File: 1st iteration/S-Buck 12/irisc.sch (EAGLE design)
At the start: 14 parts, among them U1 LM2695MH

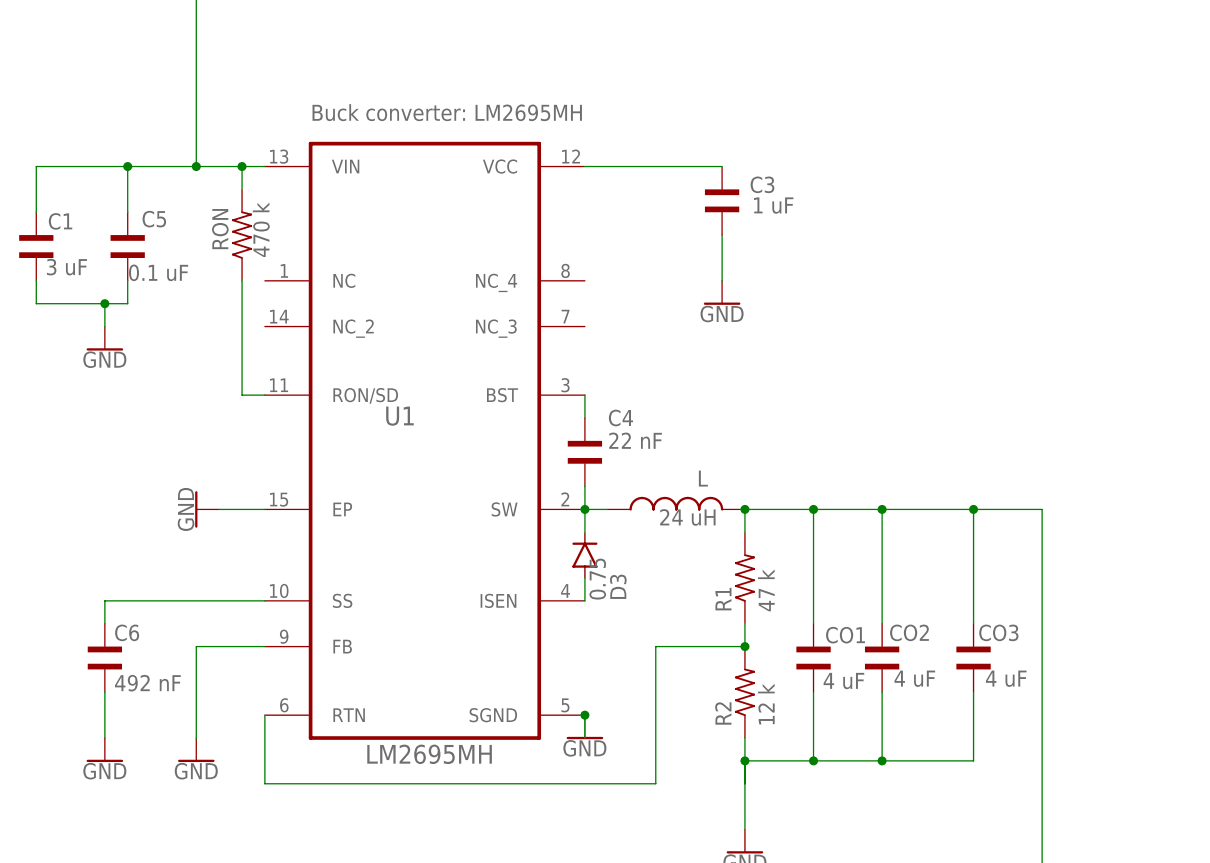
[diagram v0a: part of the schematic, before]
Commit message: Update irisc.sch
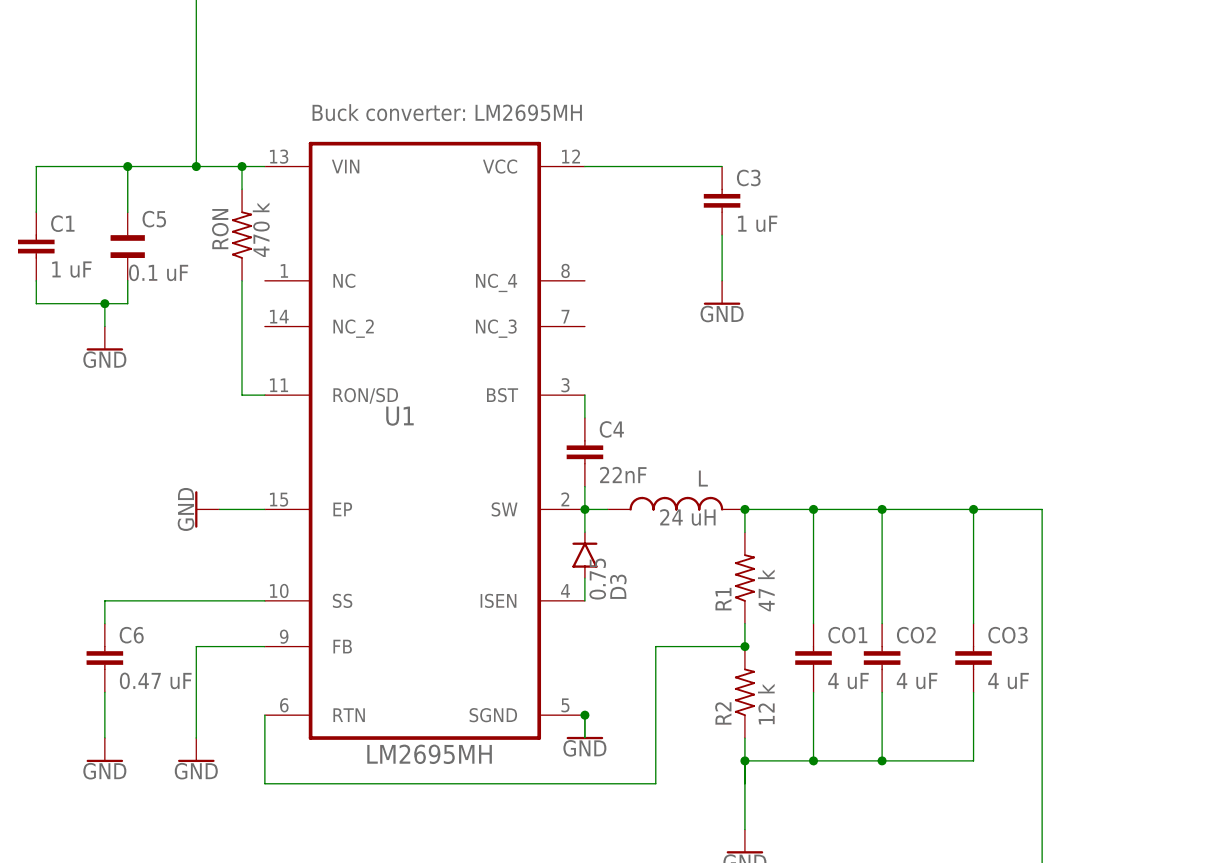
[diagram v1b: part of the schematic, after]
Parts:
- C1: value 3 uF -> 1 uF; device Wurth_Elektronik_Passive_Capacitors_rev18b:WCAP-CSGP_0805_885012006082_REFLOW -> eagle-ltspice:CC1210; SPICEPREFIX C -> (none)
- C3: device Wurth_Elektronik_Passive_Capacitors_rev18b:WCAP-CSGP_0805_885012006018_WAVE -> eagle-ltspice:CC1210; SPICEPREFIX C -> (none)
- C4: value 22 nF -> 22nF; device Wurth_Elektronik_Passive_Capacitors_rev18b:WCAP-CSGP_0805_885012006018_WAVE -> eagle-ltspice:CC1206; SPICEPREFIX C -> (none)
- C6: value 492 nF -> 0.47 uF; device Wurth_Elektronik_Passive_Capacitors_rev18b:WCAP-CSGP_0805_885012006018_WAVE -> eagle-ltspice:CC1210; SPICEPREFIX C -> (none)
- CO1, CO2, CO3: device Wurth_Elektronik_Passive_Capacitors_rev18b:WCAP-CSGP_0805_885012006018_WAVE -> eagle-ltspice:CC1812; SPICEPREFIX C -> (none)
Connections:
- net 12V: now also CO1.1, CO2.1, CO3.1; no longer CO1.2, CO2.2, CO3.2
- net GND: now also C1.2, C3.2, C6.2, CO1.2, CO2.2, CO3.2; no longer C1.1, C3.1, C6.1, CO1.1, CO2.1, CO3.1
- net N$124: now also C3.1; no longer C3.2
- net N$125: now also C4.1; no longer C4.2
- net N$126: now also C4.2; no longer C4.1
- net N$128: now also C6.1; no longer C6.2
- net VCC: now also C1.1; no longer C1.2

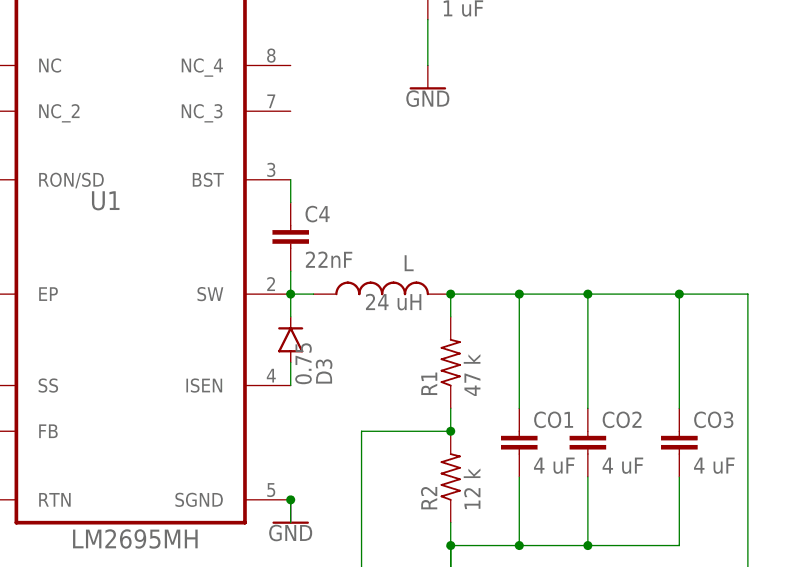
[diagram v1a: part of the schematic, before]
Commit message: Update irisc.sch
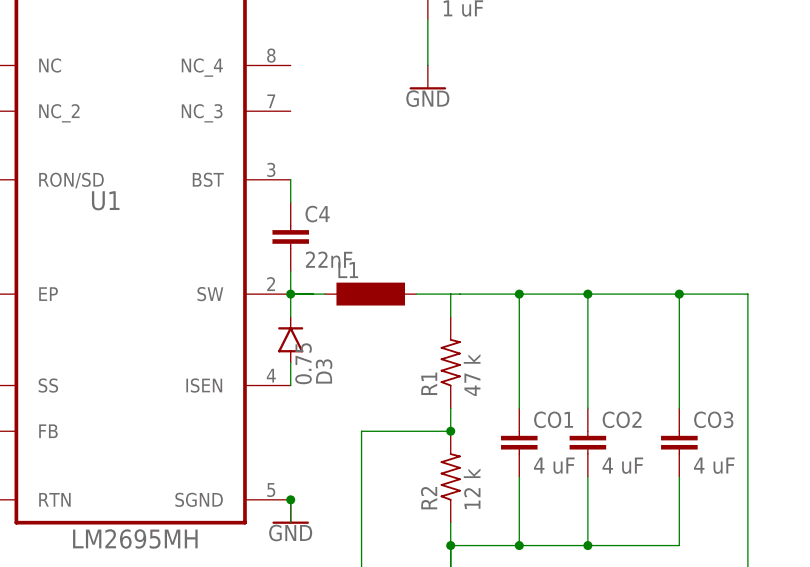
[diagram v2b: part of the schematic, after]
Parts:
- removed L: 24 uH, BeagleBone_Blue_R3:INDUCTOR
- added L1: (no value), inductor-neosid:BS11
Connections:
- net 12V: now also L1.2; no longer L.2
- net N$126: now also L1.1; no longer L.1
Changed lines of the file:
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@@
 <attribute name="SPICEPREFIX" value="R"/>
 </part>
-<part name="L" library="BeagleBone_Blue_R3" library_urn="urn:adsk.eagle:library:5828899" deviceset="INDUCTOR" device="" package3d_urn="urn:adsk.eagle:package:5829817/3" value="24 uH"/>
 <part name="D3" library="BeagleBone_Blue_R3" library_urn="urn:adsk.eagle:library:5828899" deviceset="DIODE" device="" package3d_urn="urn:adsk.eagle:package:5829545/1" value="0.75">
 <attribute name="SPICEPREFIX" value="D"/>
@@
 <part name="C6" library="eagle-ltspice" library_urn="urn:adsk.eagle:library:217" deviceset="C" device="C1210" package3d_urn="urn:adsk.eagle:package:13278/1" value="0.47 uF"/>
 <part name="C4" library="eagle-ltspice" library_urn="urn:adsk.eagle:library:217" deviceset="C" device="C1206" package3d_urn="urn:adsk.eagle:package:13279/1" value="22nF"/>
+<part name="L1" library="inductor-neosid" library_urn="urn:adsk.eagle:library:241" deviceset="BS" device="11" package3d_urn="urn:adsk.eagle:package:14648/1"/>
 </parts>
 <sheets>
@@
 <attribute name="VALUE" x="33.528" y="86.36" size="1.778" layer="96" rot="R90"/>
 </instance>
-<instance part="L" gate="G$1" x="78.74" y="58.42" smashed="yes" rot="R90">
-<attribute name="NAME" x="81.026" y="60.96" size="1.778" layer="95"/>
-<attribute name="VALUE" x="83.312" y="58.42" size="1.778" layer="96" rot="R180"/>
-</instance>
 <instance part="D3" gate="G$1" x="68.58" y="53.34" smashed="yes" rot="R90">
 <attribute name="NAME" x="73.1774" y="48.26" size="1.778" layer="95" rot="R90"/>
@@
 <attribute name="NAME" x="70.104" y="66.421" size="1.778" layer="95"/>
 <attribute name="VALUE" x="70.104" y="61.341" size="1.778" layer="96"/>
+</instance>
+<instance part="L1" gate="G$1" x="77.47" y="58.42" smashed="yes">
+<attribute name="NAME" x="73.66" y="60.198" size="1.778" layer="95"/>
+<attribute name="VALUE" x="73.66" y="54.864" size="1.778" layer="96"/>
 </instance>
 </instances>
@@
 <wire x1="68.58" y1="55.88" x2="68.58" y2="58.42" width="0.1524" layer="91"/>
 <junction x="68.58" y="58.42"/>
-<pinref part="L" gate="G$1" pin="1"/>
 <wire x1="71.12" y1="58.42" x2="68.58" y2="58.42" width="0.1524" layer="91"/>
 <pinref part="U1" gate="A" pin="SW"/>
 <pinref part="C4" gate="G$1" pin="2"/>
+<pinref part="L1" gate="G$1" pin="1"/>
+<wire x1="68.58" y1="58.42" x2="72.39" y2="58.42" width="0.1524" layer="91"/>
 </segment>
 </net>
@@
 <net name="12V" class="0">
 <segment>
-<pinref part="L" gate="G$1" pin="2"/>
 <pinref part="R1" gate="G$1" pin="2"/>
 <wire x1="86.36" y1="58.42" x2="86.36" y2="55.88" width="0.1524" layer="91"/>
-<wire x1="86.36" y1="58.42" x2="93.98" y2="58.42" width="0.1524" layer="91"/>
-<junction x="86.36" y="58.42"/>
+<wire x1="86.36" y1="58.42" x2="87.376" y2="58.42" width="0.1524" layer="91"/>
+<wire x1="87.376" y1="58.42" x2="93.98" y2="58.42" width="0.1524" layer="91"/>
 <wire x1="93.98" y1="58.42" x2="101.6" y2="58.42" width="0.1524" layer="91"/>
 <junction x="93.98" y="58.42"/>
@@
 <pinref part="CO2" gate="G$1" pin="1"/>
 <pinref part="CO3" gate="G$1" pin="1"/>
-</segment>
-</net>
+<pinref part="L1" gate="G$1" pin="2"/>
+<wire x1="82.55" y1="58.42" x2="86.36" y2="58.42" width="0.1524" layer="91"/>
+</segment>
+</net>
